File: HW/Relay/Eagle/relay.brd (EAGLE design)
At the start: 100 x 80 mm, 41 parts, among them IC2 DS18B20, K2 CQ1-12V, Q1A MMBT3904, Q1B MMBT3904, T1 BC847, U3 MCP16311

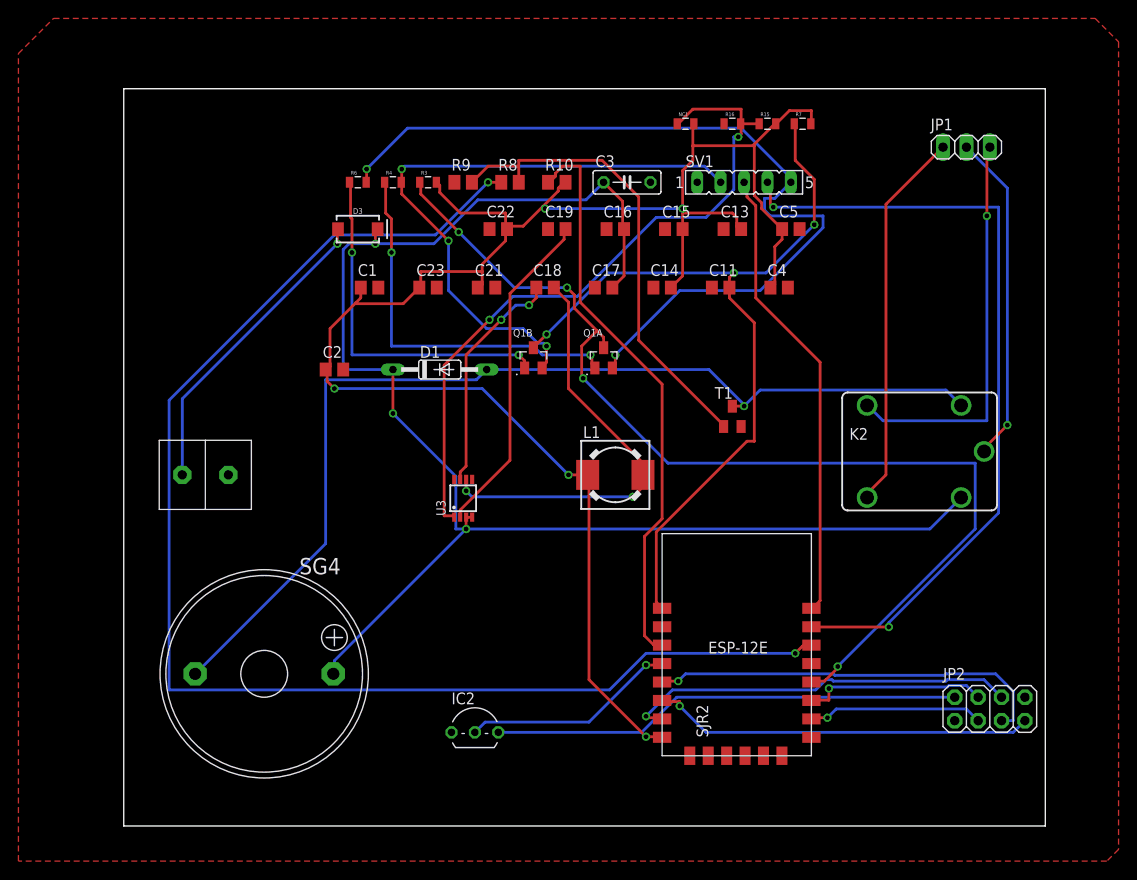
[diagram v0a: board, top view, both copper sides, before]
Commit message: Add files via upload
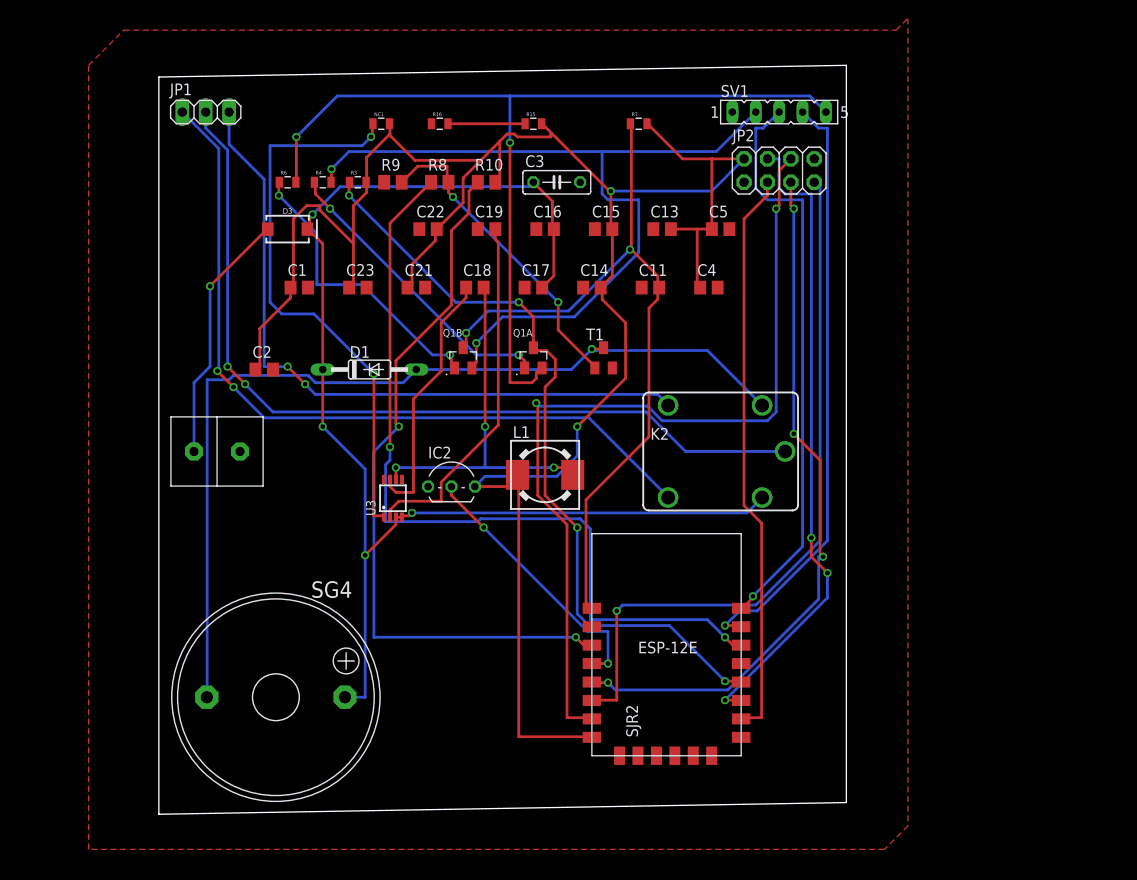
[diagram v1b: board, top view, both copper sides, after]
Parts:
- moved JP1 82.6 mm to (8.89, 77.5)
- moved JP2 62.7 mm to (71.1, 71.1)
- moved NC1 33.0 mm to (27.9, 76.2)
- moved R16 31.8 mm to (34.3, 76.2)
- moved IC2 26.8 mm to (35.6, 36.8)
- moved R15 25.4 mm to (44.5, 76.2)
- moved K2 21.6 mm to (64.8, 40.6)
- moved R7 17.8 mm to (55.9, 76.2)
- moved T1 15.3 mm to (52.1, 50.8)
- moved SV1 8.52 mm to (71.1, 77.5)
- moved C13 7.62 mm to (58.4, 64.8)
- moved C14 7.62 mm to (50.8, 58.4)
- moved C16 7.62 mm to (45.7, 64.8)
- moved C19 7.62 mm to (39.4, 64.8)
- moved C23 7.62 mm to (25.4, 58.4)
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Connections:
- new net N$3: NC1.1, U3.VFB
- net N$28: no longer NC1.1, U3.VFB
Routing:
- net N$28: track 75.8 -> 8.36 mm, vias 2 -> 0
- net N$3: track 0.00 -> 60.9 mm, vias 0 -> 2
- net RELAY_DATA: track 149.0 -> 89.1 mm
- net C: track 36.0 -> 92.9 mm, vias 1 -> 2
- net RF_MOSI: track 43.2 -> 93.7 mm, vias 1 -> 2
- net RF_CSN: track 20.0 -> 70.2 mm, vias 1 -> 3
- net RF_CE: track 19.1 -> 62.2 mm, vias 1 -> 0
- net NC: track 41.5 -> 84.5 mm, vias 0 -> 2
- net RF_MISO: track 41.7 -> 77.2 mm
- net RF_SCK: track 43.9 -> 76.2 mm, vias 1 -> 4
- net NO: track 43.5 -> 74.8 mm, vias 1 -> 2
- net PROG_IR_TR: track 113.8 -> 83.8 mm
- net RTS: track 66.5 -> 89.2 mm, vias 3 -> 2
- net VRELAY: track 164.5 -> 142.1 mm, vias 3 -> 4
- net RXD: track 86.3 -> 65.0 mm, vias 2 -> 1
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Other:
- board size 100 x 80 mm -> 74.6 x 81.3 mm

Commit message: Add files via upload
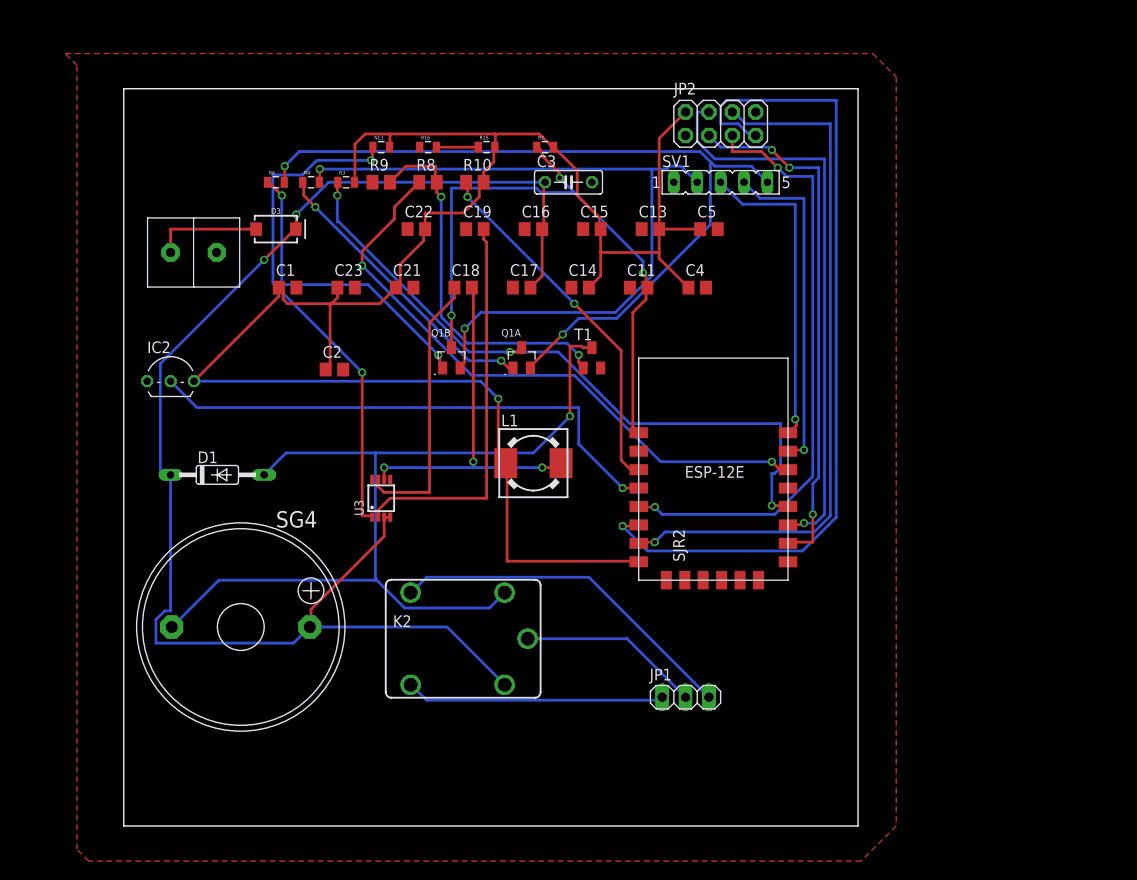
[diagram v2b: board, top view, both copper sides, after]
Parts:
- moved JP1 82.1 mm to (61.0, 14.0)
- moved K2 34.5 mm to (36.8, 20.3)
- moved IC2 32.6 mm to (5.08, 48.3)
- moved U$1 21.7 mm to (7.62, 62.2)
- moved D1 20.1 mm to (10.2, 38.1)
- moved SJR2 19.7 mm to (63.5, 36.8)
- moved R7 10.5 mm to (45.7, 73.7)
- moved SV1 9.92 mm to (64.8, 69.8)
- moved SG4 8.52 mm to (12.7, 21.6)
- moved JP2 8.13 mm to (64.8, 76.2)
- moved C2 7.62 mm to (22.9, 49.5)
- moved R15 5.68 mm to (39.4, 73.7)
- moved R16 2.84 mm to (33.0, 73.7)
- moved NC1 2.54 mm to (27.9, 73.7)
- moved L1 1.80 mm to (44.5, 39.4)
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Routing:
- net C: track 92.9 -> 19.8 mm, vias 2 -> 0
- net NC: track 84.5 -> 28.1 mm, vias 2 -> 0
- net N$30: track 78.4 -> 39.6 mm
- net NO: track 74.8 -> 38.4 mm, vias 2 -> 0
- net RXD: track 65.0 -> 36.3 mm
- net DS18B20: track 29.3 -> 57.9 mm, vias 2 -> 1
- net TXD: track 62.5 -> 34.4 mm
- net VCC: track 234.5 -> 206.9 mm, vias 2 -> 1
- net RELAY_DATA: track 89.1 -> 67.0 mm
- net RF_MOSI: track 93.7 -> 75.8 mm, vias 2 -> 1
- net VIN: track 27.5 -> 11.8 mm, vias 1 -> 0
- net RF_MISO: track 77.2 -> 92.0 mm
- net RESET: track 80.9 -> 67.8 mm, vias 2 -> 3
- net DTR: track 100.6 -> 89.1 mm
- net RF_SCK: track 76.2 -> 65.1 mm, vias 4 -> 2
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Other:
- board size 74.6 x 81.3 mm -> 79.7 x 80 mm
